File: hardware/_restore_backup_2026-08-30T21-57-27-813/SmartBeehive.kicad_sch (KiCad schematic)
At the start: 7 parts, among them U2 HX711_Module, U3 SSD1306, U4 DS18B20, U5 INMP441, U6 SHT31

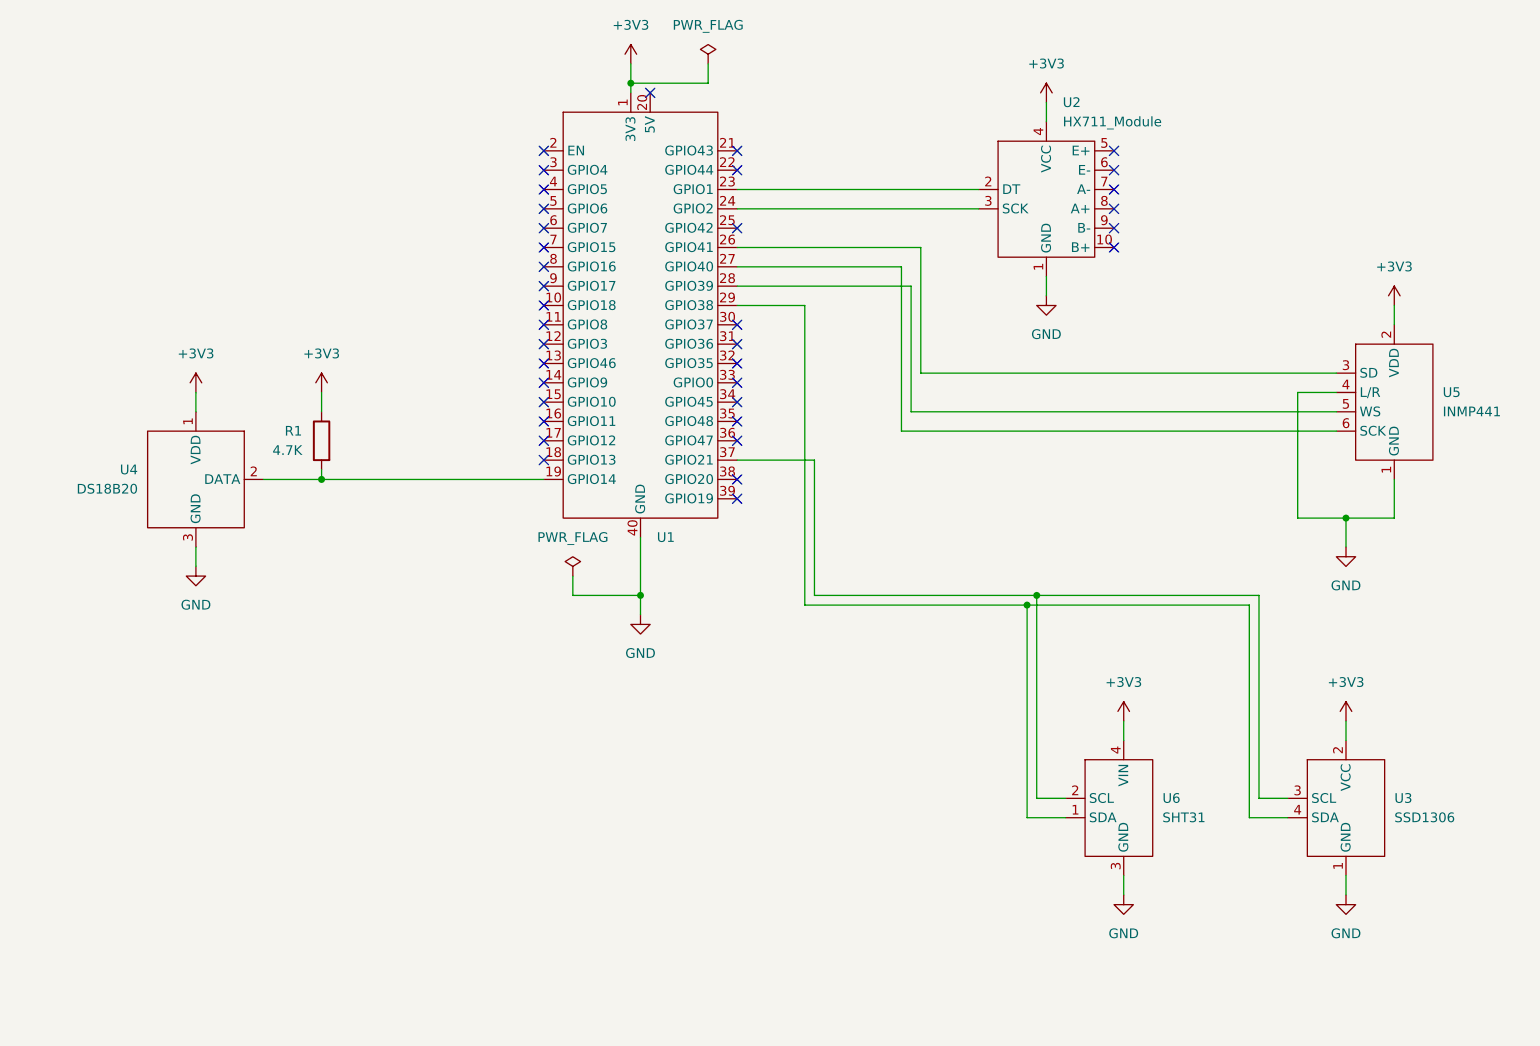
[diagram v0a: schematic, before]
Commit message: Refactor code structure for improved readability and maintainability
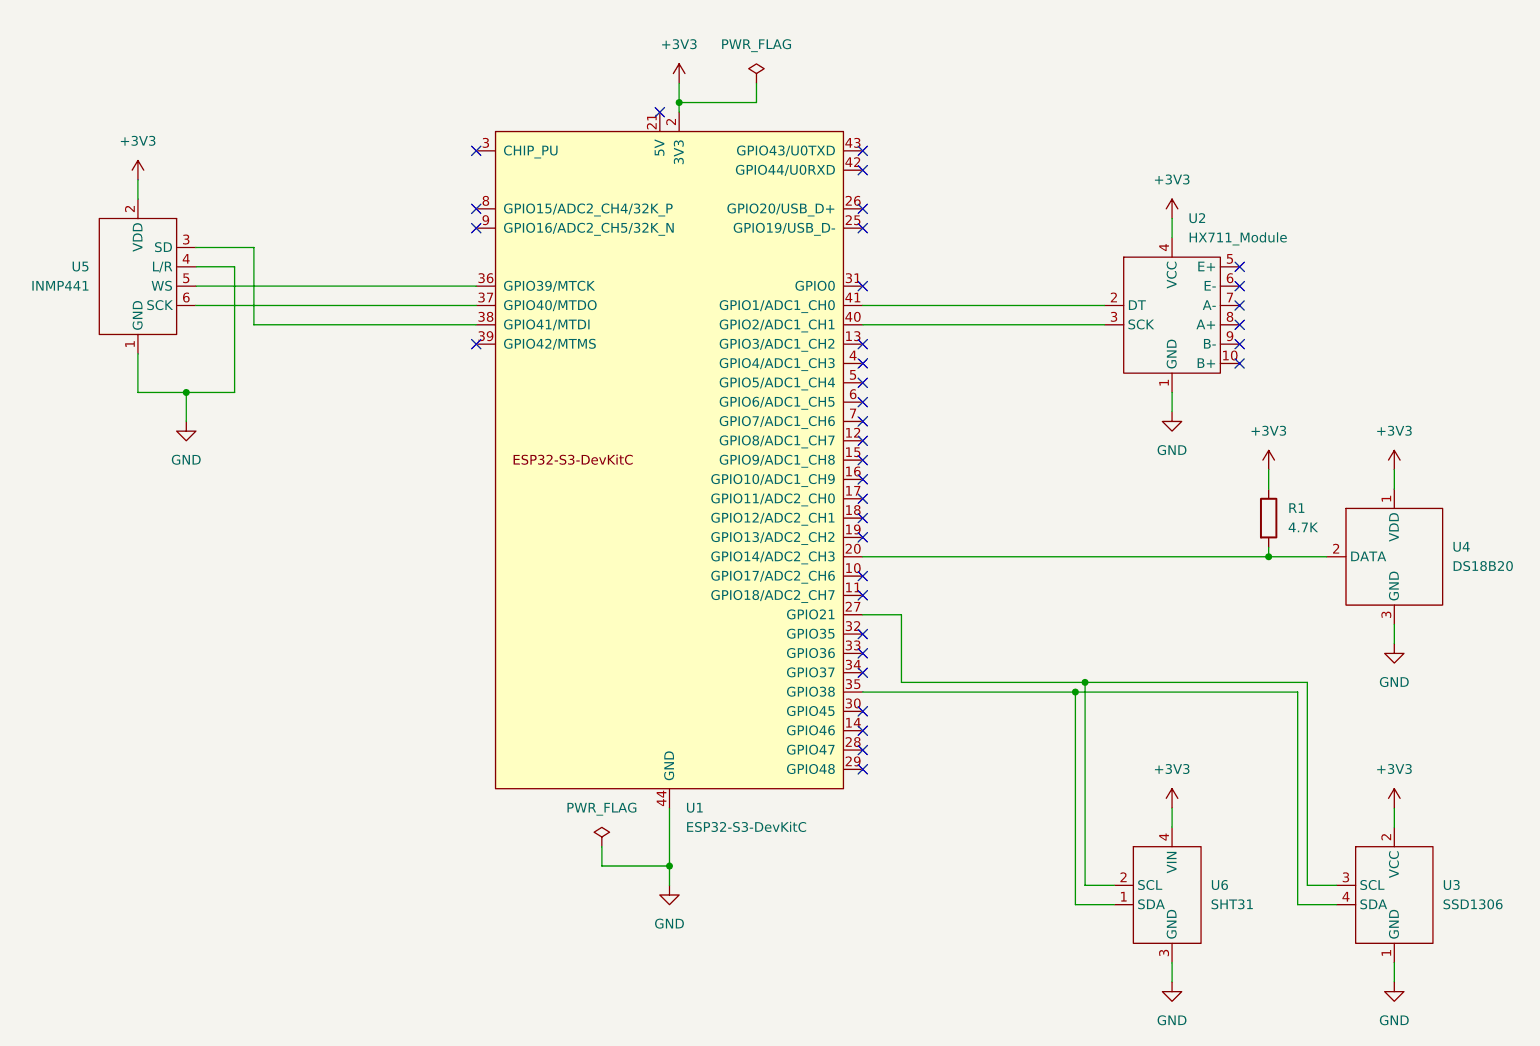
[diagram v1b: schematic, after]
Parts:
- removed U1: (no value), SmartBeehiveLib:Freenove_ESP32_S3, symbol HX711_BreakOut:Freenove_ESP32_S3
- added U1: ESP32-S3-DevKitC, PCM_Espressif:ESP32-S3-DevKitC, symbol PCM_Espressif:ESP32-S3-DevKitC
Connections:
- net +3V3: now also U1.1 (3V3), U1.2 (3V3)
- net GND: now also U1.22 (GND), U1.23 (GND), U1.24 (GND), U1.44 (GND)
- net at R1.2, U4.2 (DATA): now also U1.20 (GPIO14/ADC2_CH3)
- net at U2.2 (DT): now also U1.41 (GPIO1/ADC1_CH0)
- net at U2.3 (SCK): now also U1.40 (GPIO2/ADC1_CH1)
- net at U5.3 (SD): now also U1.38 (GPIO41/MTDI)
- net at U5.6 (SCK): now also U1.37 (GPIO40/MTDO)
- net at U5.5 (WS): now also U1.36 (GPIO39/MTCK)
- net at U3.4 (SDA), U6.1 (SDA): now also U1.35 (GPIO38)
- net at U3.3 (SCL), U6.2 (SCL): now also U1.27 (GPIO21)
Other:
- moved on the sheet: R1, U2, U3, U4, U5, U6
